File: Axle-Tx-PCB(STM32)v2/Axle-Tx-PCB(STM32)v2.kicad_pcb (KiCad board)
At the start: 2 copper layers, 36.7 x 18.5 mm, 21 parts, among them J1 SWD Con, J2 nRF24L01 Con

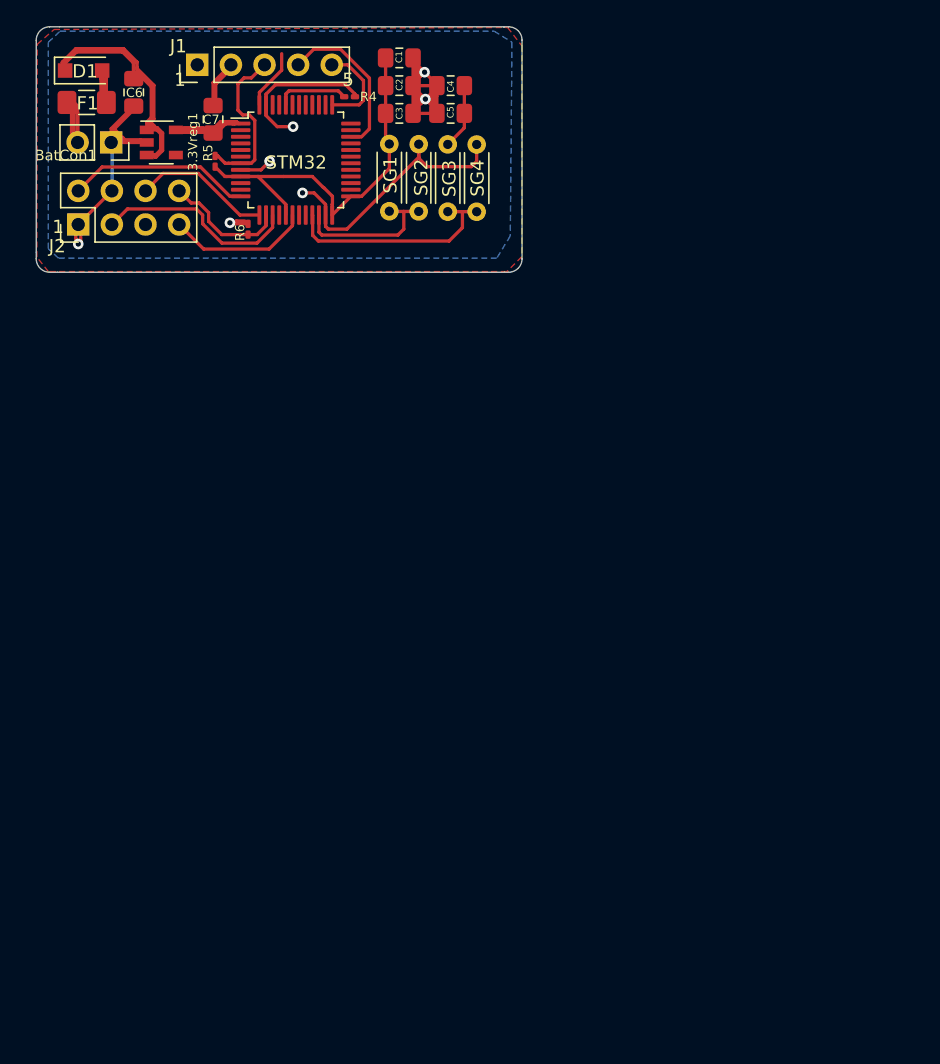
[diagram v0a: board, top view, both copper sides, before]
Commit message: final versions of PCBs, ordered through JLCPCB 2020-12-30
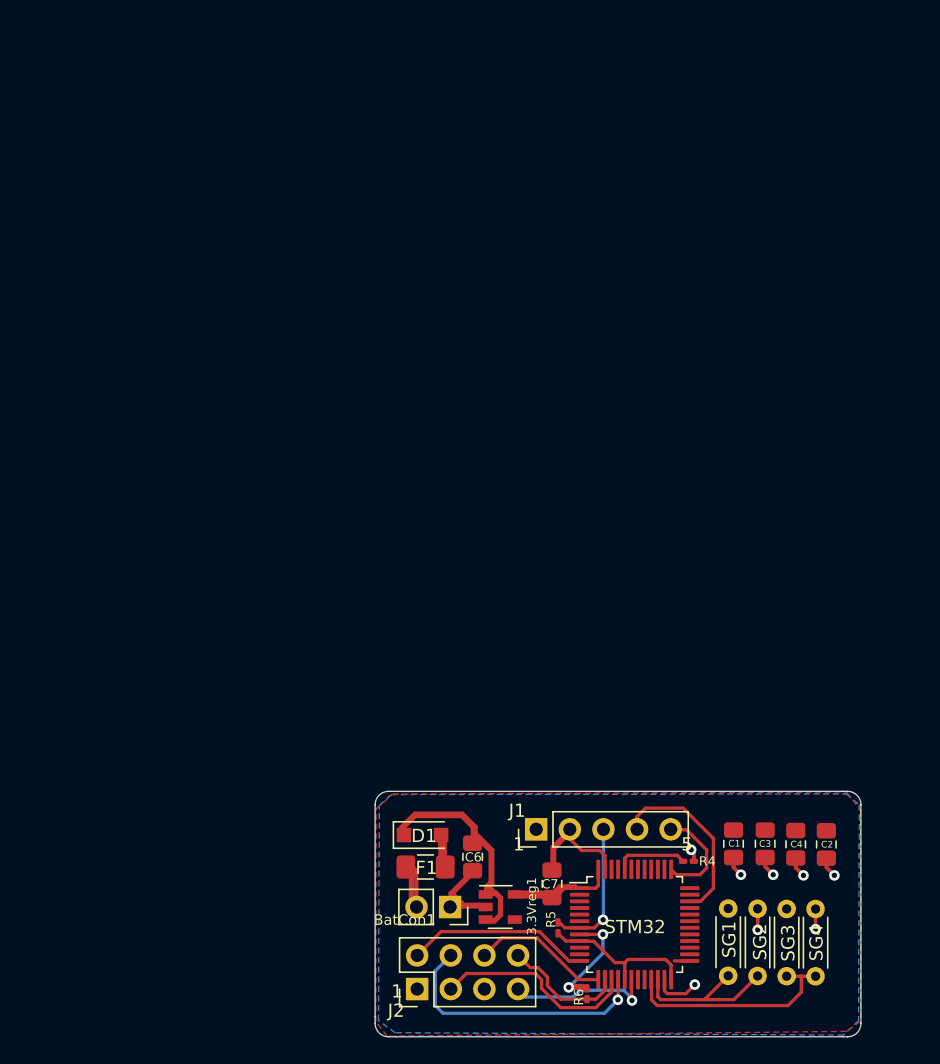
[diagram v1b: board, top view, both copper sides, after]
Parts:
- removed C5: 10nF, Capacitor_SMD:C_0805_2012Metric_Pad1.18x1.45mm_HandSolder
- moved C2 65.8 mm to (62.4, 40.5), turned to 270 degrees
- moved C1 64.5 mm to (55.4, 40.4), turned to 270 degrees
- moved R5 63.4 mm to (42.2, 46.8)
- moved 3.3Vreg1 63.2 mm to (37.8, 45.2)
- moved BatCon1 63.2 mm to (34.0, 45.2)
- moved D1 63.2 mm to (31.9, 39.8)
- moved STM32 63.2 mm to (48.0, 46.5)
- moved C6 63.2 mm to (35.7, 41.4)
- moved C7 63.2 mm to (41.7, 43.5)
- moved F1 63.2 mm to (32.2, 42.2)
- moved J1 63.2 mm to (40.5, 39.3)
- moved J2 63.2 mm to (31.5, 51.4)
- moved R6 63.2 mm to (44.3, 51.8)
- moved SG1 63.2 mm to (55.0, 45.3)
- moved SG2 63.2 mm to (57.2, 50.4)
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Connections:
- 3.3Vreg1 pad 2: SPI1-MISO -> GND
- 3.3Vreg1 pad 5: VBAT -> +3V3
- BatCon1 pad 1: SPI1-MISO -> GND
- C1 pad 2: SPI1-MISO -> GND
- C2 pad 2: SPI1-MISO -> GND
- C3 pad 2: SPI1-MISO -> GND
- C4 pad 2: SPI1-MISO -> GND
- C6 pad 2: SPI1-MISO -> GND
- C7 pad 1: VBAT -> +3V3
- C7 pad 2: SPI1-MISO -> GND
- J1 pad 2: SPI1-MISO -> GND
- J2 pad 1: SPI1-MISO -> GND
- R4 pad 2: SPI1-MISO -> GND
- R6 pad 1: SPI1-MISO -> GND
- SG2 pad 2: SPI1-MISO -> GND
- SG4 pad 2: SPI1-MISO -> GND
- STM32 pad 1: VBAT -> +3V3
- STM32 pad 16: Net-(STM32-Pad16) -> SPI1-MISO
- STM32 pad 23: SPI1-MISO -> GND
- STM32 pad 47: SPI1-MISO -> GND
- STM32 pad 8: SPI1-MISO -> GND
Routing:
- net SPI1-MISO: track 98.9 -> 23.1 mm, vias 7 -> 1
- net GND: track 0.00 -> 48.4 mm, vias 0 -> 10
- net VBAT: track 13.6 -> 0.00 mm
- net +3V3: track 39.0 -> 29.7 mm
- net NRST: track 12.5 -> 10.8 mm, vias 0 -> 1
- net PA13-SWDIO: track 12.3 -> 13.9 mm
- net PA14-SWCLK: track 6.93 -> 7.84 mm
- net SDADC-AIN8m: track 11.5 -> 12.2 mm
- net SPI1-MOSI: track 10.9 -> 11.1 mm, vias 0 -> 1
- added copper zone on B.Cu, net GND
- removed copper zone on B.Cu, net SPI1-MISO

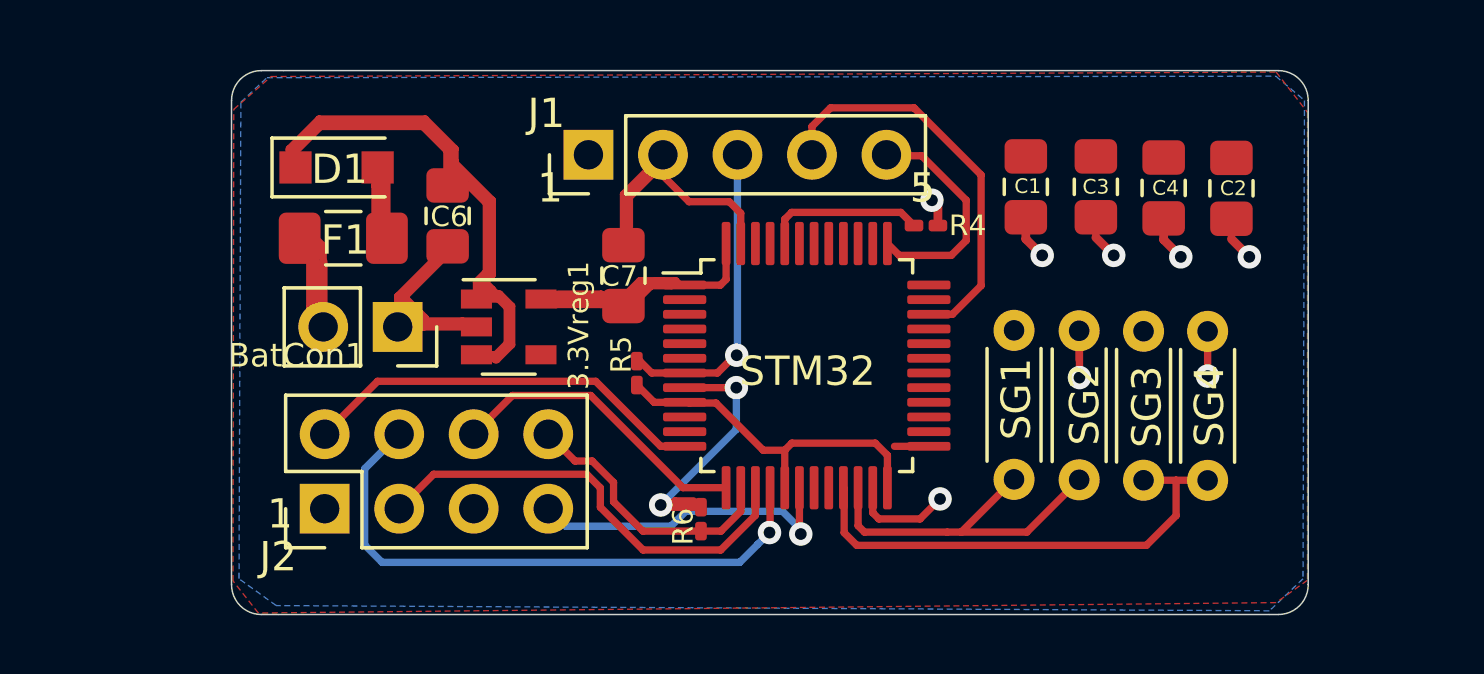
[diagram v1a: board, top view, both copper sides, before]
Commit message: PCB's ready for final review before order
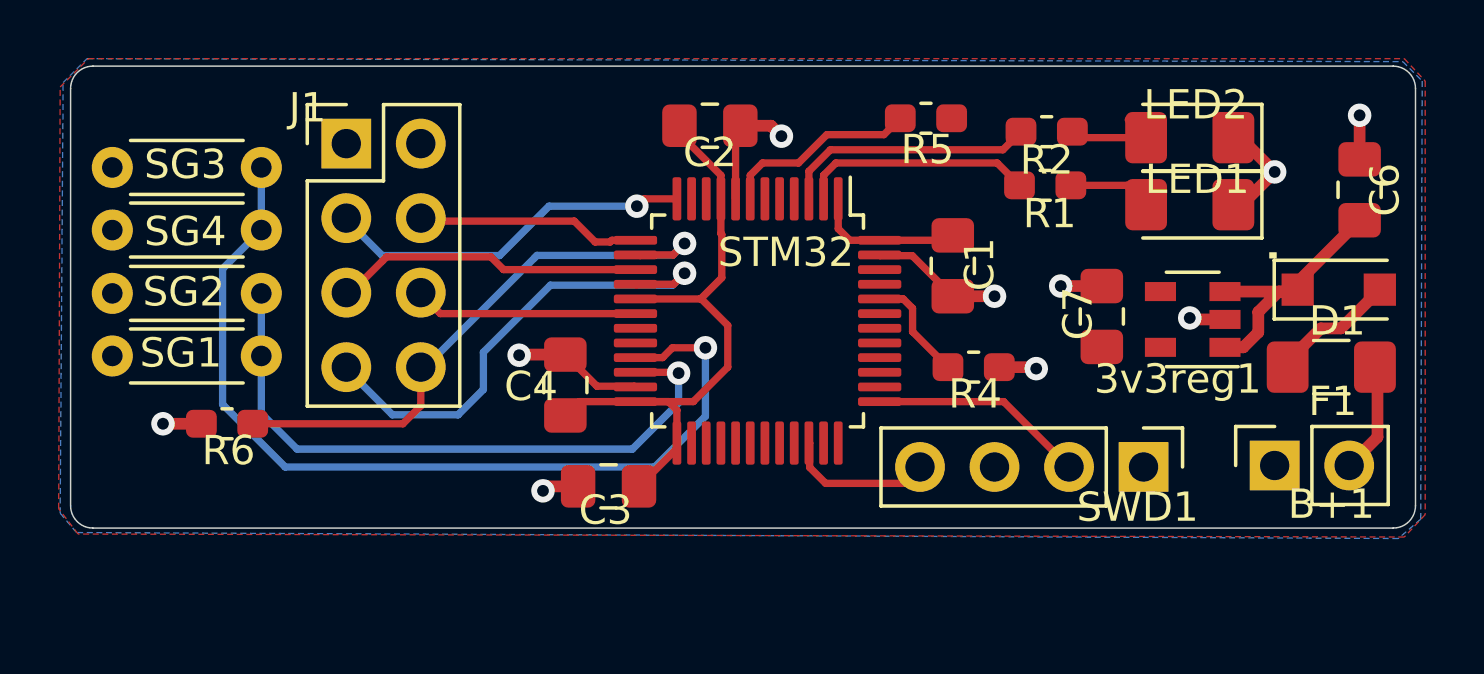
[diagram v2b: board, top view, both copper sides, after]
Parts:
- removed 3.3Vreg1: LD39015M33R, Package_TO_SOT_SMD:SOT-23-5
- removed BatCon1: 4P2C, Connector_PinSocket_2.54mm:PinSocket_1x02_P2.54mm_Vertical
- removed J2: nRF24L01 Con, Connector_PinHeader_2.54mm:PinHeader_2x04_P2.54mm_Vertical
- added 3v3reg1: LD39015M33R, Package_TO_SOT_SMD:SOT-23-5, F.Cu at (61.1, 45.0)
- added B+1: 4P2C, Connector_PinSocket_2.54mm:PinSocket_1x02_P2.54mm_Vertical, F.Cu at (63.9, 49.9)
- added LED1: LED, LED_SMD:LED_1206_3216Metric_Pad1.42x1.75mm_HandSolder, F.Cu at (61.0, 41.0)
- added LED2: LED, LED_SMD:LED_1206_3216Metric_Pad1.42x1.75mm_HandSolder, F.Cu at (61.0, 38.8)
- added R1: 2k2, Resistor_SMD:R_0603_1608Metric_Pad1.05x0.95mm_HandSolder, F.Cu at (56.1, 40.4)
- added R2: 2k2, Resistor_SMD:R_0603_1608Metric_Pad1.05x0.95mm_HandSolder, F.Cu at (56.1, 38.6)
- added SWD1: SWDConnector, Connector_PinHeader_2.54mm:PinHeader_1x04_P2.54mm_Vertical, F.Cu at (59.4, 50.0)
- J1: value SWD Con -> nRF24; footprint Connector_PinHeader_2.54mm:PinHeader_1x05_P2.54mm_Vertical -> Connector_PinHeader_2.54mm:PinHeader_2x04_P2.54mm_Vertical
- R4, R5, R6: footprint Resistor_SMD:R_0201_0603Metric_Pad0.64x0.40mm_HandSolder -> Resistor_SMD:R_0603_1608Metric_Pad1.05x0.95mm_HandSolder
- moved SG3 35.6 mm to (24.3, 39.8), turned to 0 degrees
- moved D1 34.4 mm to (66.1, 43.9)
- moved F1 34.0 mm to (65.8, 46.6), turned to 0 degrees
- moved SG4 33.4 mm to (29.4, 41.9), turned to 180 degrees
- moved C6 31.1 mm to (66.8, 40.5), turned to 90 degrees
- moved SG1 30.8 mm to (24.3, 46.2), turned to 0 degrees
- moved SG2 28.6 mm to (29.4, 44.1), turned to 180 degrees
- moved C4 21.5 mm to (39.7, 47.2), turned to 90 degrees
- moved C3 19.5 mm to (41.2, 50.6), turned to 180 degrees
- moved C2 17.9 mm to (44.7, 38.4), turned to 0 degrees
- moved R6 16.5 mm to (28.2, 48.5), turned to 0 degrees
- moved C7 16.4 mm to (58.0, 44.9)
- moved R5 13.1 mm to (52.0, 38.1), turned to 180 degrees
- moved J1 8.26 mm to (32.3, 39.0), turned to 0 degrees
- moved R4 5.09 mm to (53.6, 46.6)
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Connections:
- J1 pad 1: +3V3 -> GND
- J1 pad 2: GND -> +3V3
- J1 pad 3: NRST -> SPI1-CE
- J1 pad 4: PA13-SWDIO -> SPI1-CSn
- J1 pad 5: PA14-SWCLK -> SPI1-SCK
- R5 pad 2: NRST -> Net-(R5-Pad2)
- STM32 pad 7: NRST -> Net-(R5-Pad2)
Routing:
- net Net-(3v3reg1-Pad1): track 34.6 -> 9.24 mm
- net GND: track 48.4 -> 25.4 mm
- net SDADC1-AIN8p: track 16.8 -> 31.5 mm, vias 0 -> 1
- net NRST: track 10.8 -> 0.00 mm, vias 1 -> 0
- net SPI1-IRQ: track 9.40 -> 20.0 mm, vias 0 -> 1
- net SDADC-AIN8m: track 12.2 -> 22.0 mm, vias 0 -> 1
- net PA13-SWDIO: track 13.9 -> 5.07 mm
- net Net-(R2-Pad1): track 0.00 -> 8.73 mm
- net Net-(R1-Pad1): track 0.00 -> 7.97 mm
- net Net-(R5-Pad2): track 0.00 -> 6.77 mm
- net SPI1-MISO: track 23.1 -> 16.7 mm
- net Net-(B+1-Pad2): track 9.35 -> 3.79 mm
- net SPI1-SCK: track 15.5 -> 10.5 mm
- net SPI1-MOSI: track 11.1 -> 7.52 mm, vias 1 -> 0
- net Net-(LED2-Pad2): track 0.00 -> 3.46 mm
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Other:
- board size 36.7 x 18.5 mm -> 45.8 x 15.7 mm
- board text added: "."
- board text removed: "1"
- board text removed: "5"
